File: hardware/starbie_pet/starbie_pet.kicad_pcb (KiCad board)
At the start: 2 copper layers, 11 parts, among them J1 Conn_01x04_Pin, J2 Conn_01x08_Pin, SW1 SW_Push, SW2 SW_Push, U1 XIAO-ESP32-C3-SMD, U2 DHT11

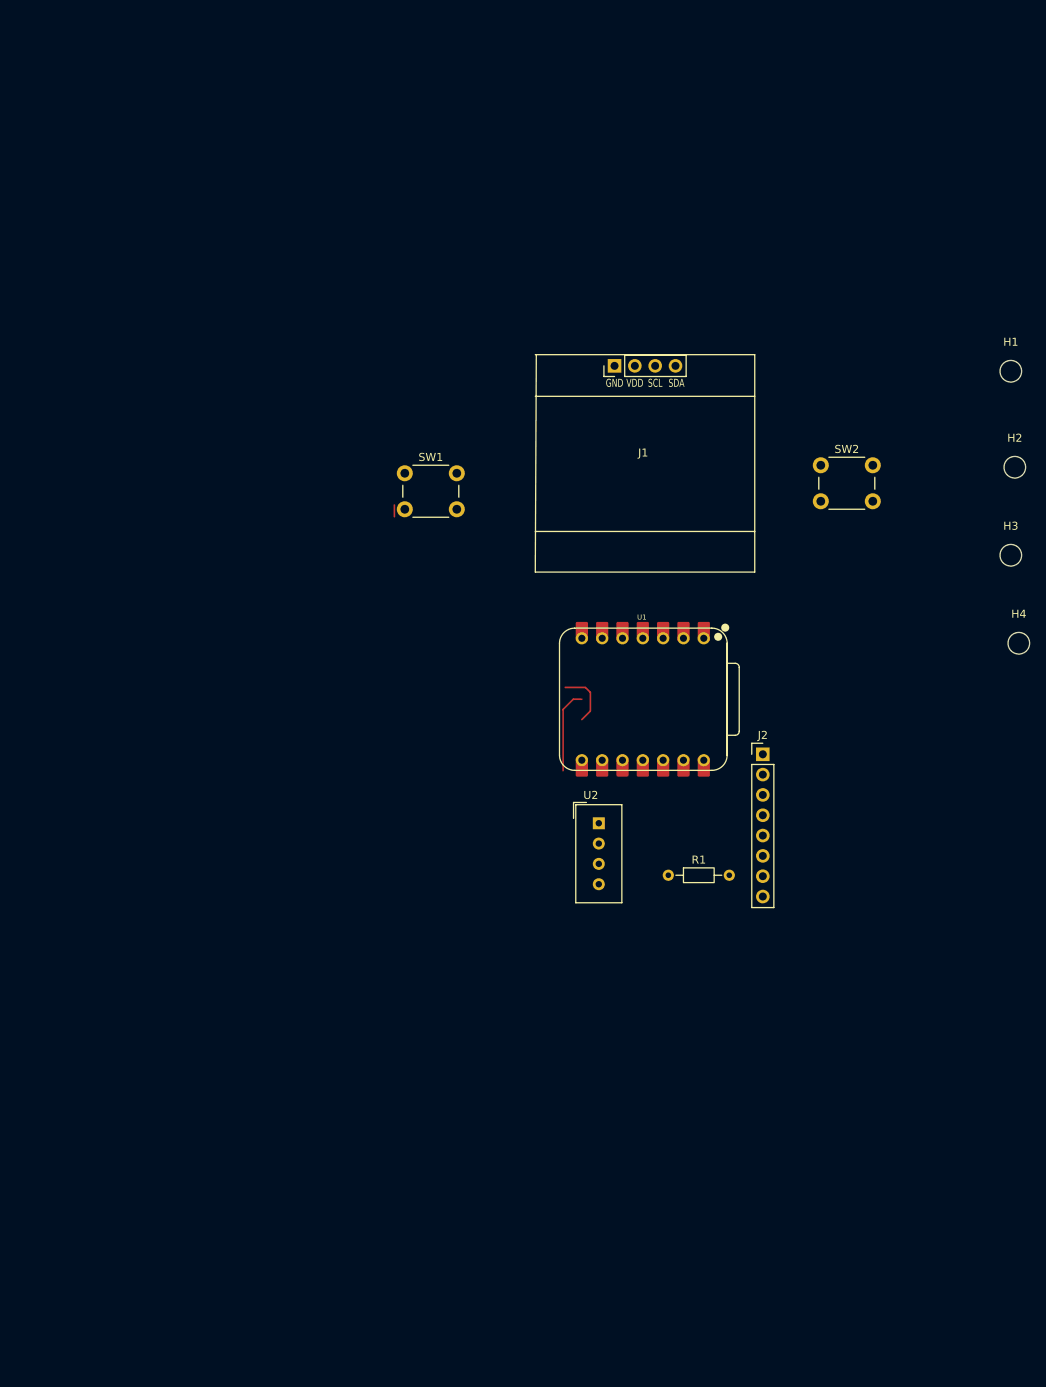
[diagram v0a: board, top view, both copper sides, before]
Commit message: before scaling
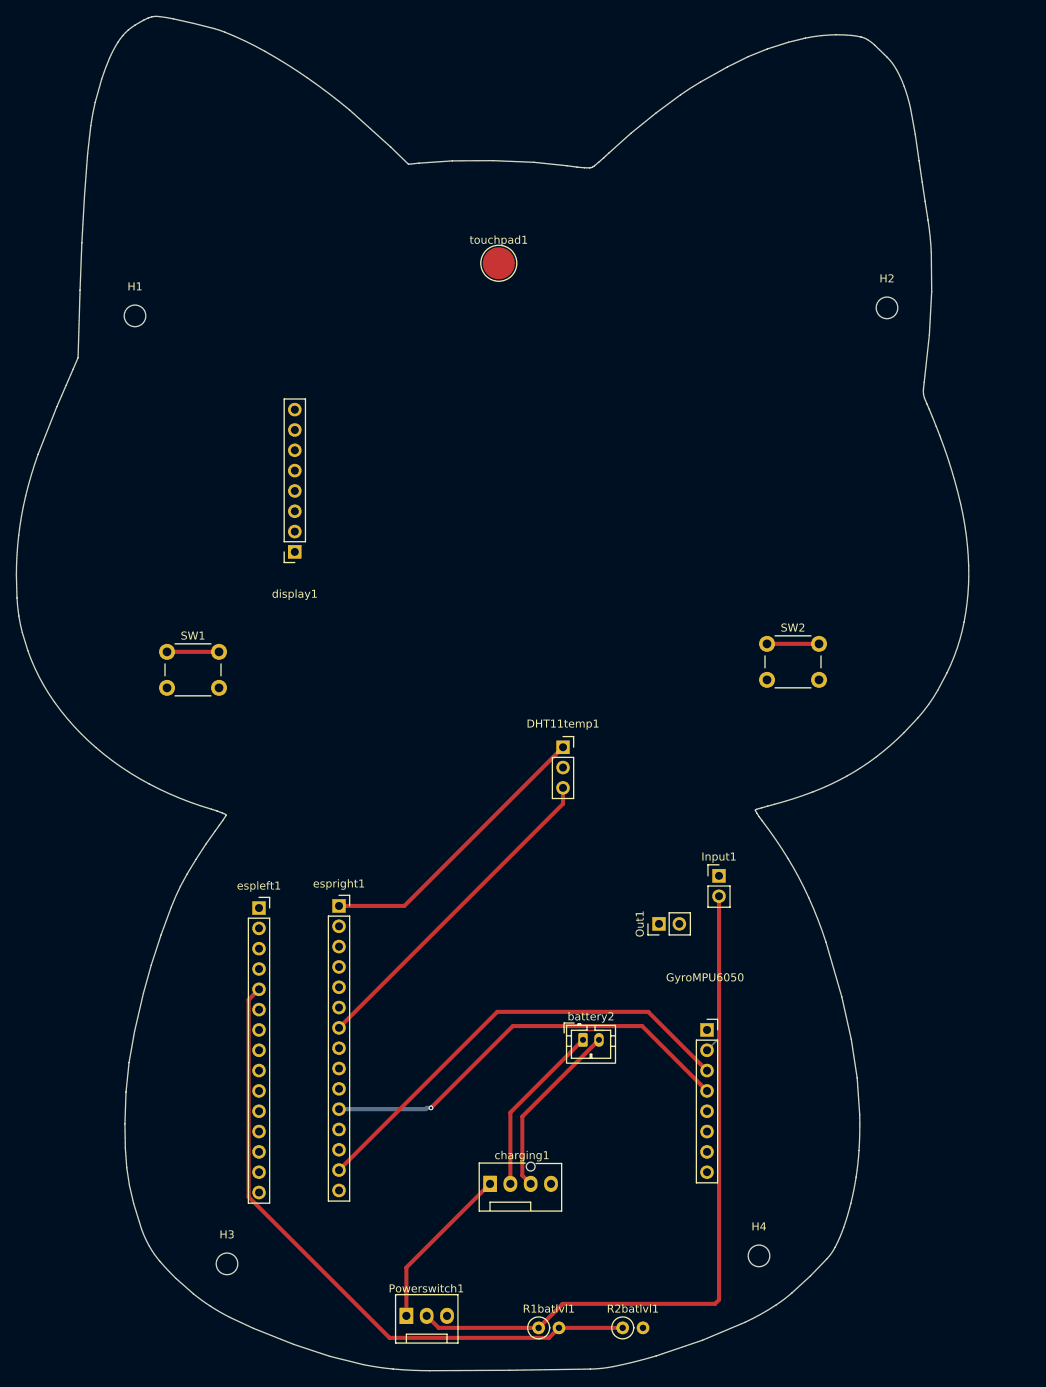
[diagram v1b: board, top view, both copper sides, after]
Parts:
- removed J1: Conn_01x04_Pin, Imported Parts:Display_128x64_096_I2C
- removed J2: Conn_01x08_Pin, Connector_PinHeader_2.54mm:PinHeader_1x08_P2.54mm_Vertical
- removed R1: 10k, Resistor_THT:R_Axial_DIN0204_L3.6mm_D1.6mm_P7.62mm_Horizontal
- removed U1: XIAO-ESP32-C3-SMD, Seeed_Studio_XIAO_Series:XIAO-ESP32-C6-DIP
- removed U2: DHT11, Sensor:Aosong_DHT11_5.5x12.0_P2.54mm
- added DHT11temp1: Conn_01x03_Socket, Connector_PinSocket_2.54mm:PinSocket_1x03_P2.54mm_Vertical, F.Cu at (134.0, 111.0)
- added GyroMPU6050: Conn_01x08_Socket, Connector_PinSocket_2.54mm:PinSocket_1x08_P2.54mm_Vertical, F.Cu at (152.0, 146.3)
- added Input1: Conn_01x02_Socket, Connector_PinHeader_2.54mm:PinHeader_1x02_P2.54mm_Vertical, F.Cu at (153.5, 127.1)
- added Out1: Conn_01x02_Socket, Connector_PinHeader_2.54mm:PinHeader_1x02_P2.54mm_Vertical, F.Cu at (146.0, 133.1)
- added Powerswitch1: SW_SPST, Connector:FanPinHeader_1x03_P2.54mm_Vertical, F.Cu at (114.4, 182.1)
- added R1batlvl1: R, Resistor_THT:R_Axial_DIN0207_L6.3mm_D2.5mm_P2.54mm_Vertical, F.Cu at (131.0, 183.6)
- added R2batlvl1: R, Resistor_THT:R_Axial_DIN0207_L6.3mm_D2.5mm_P2.54mm_Vertical, F.Cu at (141.5, 183.6)
- added battery2: Conn_01x02_Socket, Connector_JST:JST_PH_B2B-PH-K_1x02_P2.00mm_Vertical, F.Cu at (136.5, 147.6)
- added charging1: Conn_01x04_Socket, Connector:FanPinHeader_1x04_P2.54mm_Vertical, F.Cu at (124.9, 165.6)
- added display1: Conn_01x08_Socket, Connector_PinSocket_2.54mm:PinSocket_1x08_P2.54mm_Vertical, F.Cu at (100.5, 86.6)
- added espleft1: Conn_01x15_Socket, Connector_PinSocket_2.54mm:PinSocket_1x15_P2.54mm_Vertical, F.Cu at (96.0, 131.1)
- added espright1: Conn_01x15_Socket, Connector_PinSocket_2.54mm:PinSocket_1x15_P2.54mm_Vertical, F.Cu at (106.0, 130.8)
- added touchpad1: Conn_01x01, TestPoint:TestPoint_Pad_D4.0mm, F.Cu at (126.0, 50.5)
- SW1, SW2: footprint Button_Switch_THT:SW_PUSH_6mm_H5mm -> Button_Switch_THT:SW_PUSH_6mm
- moved H3 132.1 mm to (92.0, 175.6)
- moved H1 109.7 mm to (80.5, 57.1)
- moved H4 83.2 mm to (158.5, 174.6)
- moved SW1 37.2 mm to (84.5, 99.1)
- moved H2 25.5 mm to (174.5, 56.1)
- moved SW2 23.3 mm to (159.5, 98.1)
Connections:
- SW1 pad 1: GND -> /BUTTON
- SW1 pad 2: Net-(U1-D2) -> GND
- SW2 pad 1: GND -> /Button2
- SW2 pad 2: Net-(U1-D1) -> GND
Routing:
- net /Vbat: track 0.00 -> 89.1 mm
- net /Bat_sense: track 0.00 -> 81.1 mm
- net /I2C_SCL: track 0.00 -> 57.2 mm
- net /I2C_SDA: track 0.00 -> 53.7 mm, vias 0 -> 1
- net /DHT_DATA: track 0.00 -> 41.6 mm
- net +3V3: track 0.00 -> 36.2 mm
- net /Bat_neg: track 0.00 -> 22.4 mm
- net /Bat_pos: track 0.00 -> 21.8 mm
- net /CHG_OUT: track 0.00 -> 20.8 mm
- net /DHT11 DATA: track 10.5 -> 0.00 mm
- net +3.3V: track 7.25 -> 0.00 mm
- net /Button2: track 0.00 -> 6.50 mm
- net /BUTTON: track 0.00 -> 6.50 mm
- net +5V: track 0.00 -> 3.26 mm
- net GND: track 0.00 -> 1.63 mm
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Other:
- board outline added: 119.1 x 169.3 mm

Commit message: Add PCB files
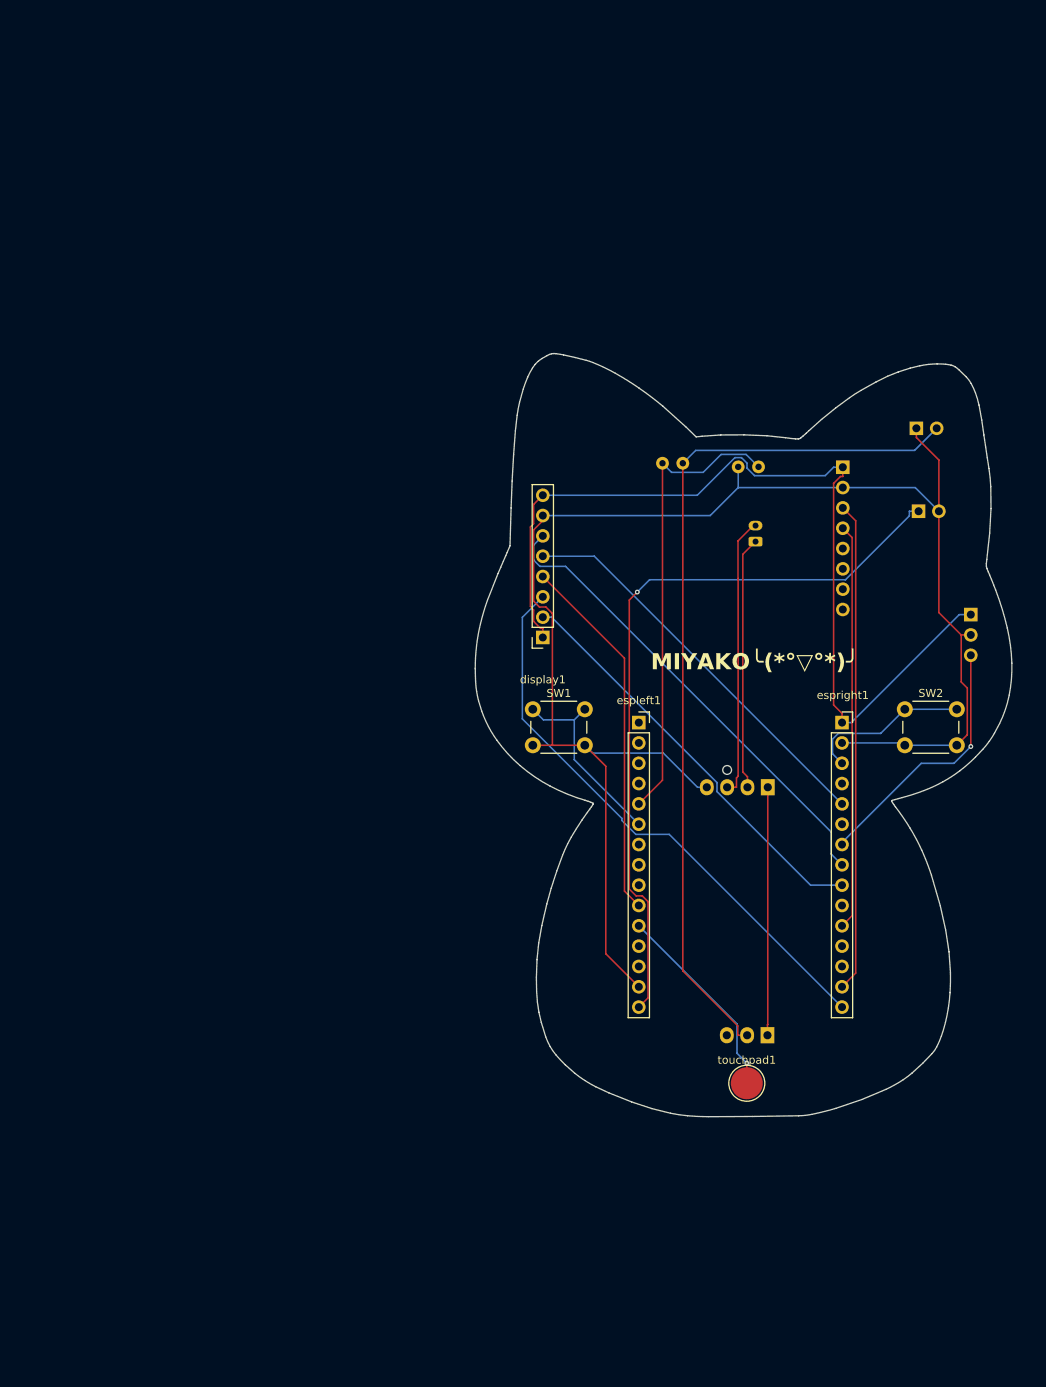
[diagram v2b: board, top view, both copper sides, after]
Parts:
- removed H1, H2, H3, H4: MountingHole, MountingHole:MountingHole_2.7mm_M2.5
- DHT11temp1, GyroMPU6050, Input1, Out1, Powerswitch1, R1batlvl1, R2batlvl1, battery2, charging1: moved to B.Cu
- moved R1batlvl1 109.6 mm to (149.0, 75.5), turned to 180 degrees
- moved R2batlvl1 109.0 mm to (158.5, 76.0), turned to 180 degrees
- moved touchpad1 107.1 mm to (157.0, 153.0)
- moved GyroMPU6050 72.4 mm to (169.0, 76.0), turned to 180 degrees
- moved espright1 66.9 mm to (168.9, 107.9)
- moved battery2 65.9 mm to (158.1, 85.3), turned to 90 degrees
- moved Input1 61.1 mm to (178.2, 71.1), turned to -90 degrees
- moved Out1 60.9 mm to (178.5, 81.5), turned to -90 degrees
- moved charging1 60.5 mm to (159.6, 116.0), turned to 180 degrees
- moved Powerswitch1 57.2 mm to (159.6, 147.0), turned to 180 degrees
- moved DHT11temp1 53.6 mm to (185.0, 94.4), turned to 180 degrees
- moved espleft1 52.8 mm to (143.5, 107.9)
- moved SW1 46.3 mm to (130.2, 106.2)
- moved display1 32.8 mm to (131.5, 97.3)
- moved SW2 19.1 mm to (176.8, 106.2)
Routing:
- net GND: track 1.63 -> 200.8 mm
- net +5V: track 3.26 -> 93.9 mm, vias 0 -> 1
- net +3V3: track 36.2 -> 115.1 mm
- net /SPI_MOSI: track 0.00 -> 71.3 mm
- net /TFT_CS: track 0.00 -> 59.5 mm
- net /SPI_CLK: track 0.00 -> 51.9 mm
- net /TFT_RST: track 0.00 -> 50.2 mm
- net /TFT_DC: track 0.00 -> 46.1 mm
- net /TOUCH: track 0.00 -> 25.3 mm, vias 0 -> 1
- net /Bat_sense: track 81.1 -> 57.9 mm
- net /Vbat: track 89.1 -> 109.1 mm
- net /BUTTON: track 6.50 -> 24.0 mm
- net /Button2: track 6.50 -> 20.6 mm
- net /Bat_neg: track 22.4 -> 35.0 mm
- net /CHG_OUT: track 20.8 -> 31.0 mm
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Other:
- board size 119.1 x 169.3 mm -> 67.1 x 95.4 mm
- board text added: "MIYAKO╰(*°▽°*)╯"

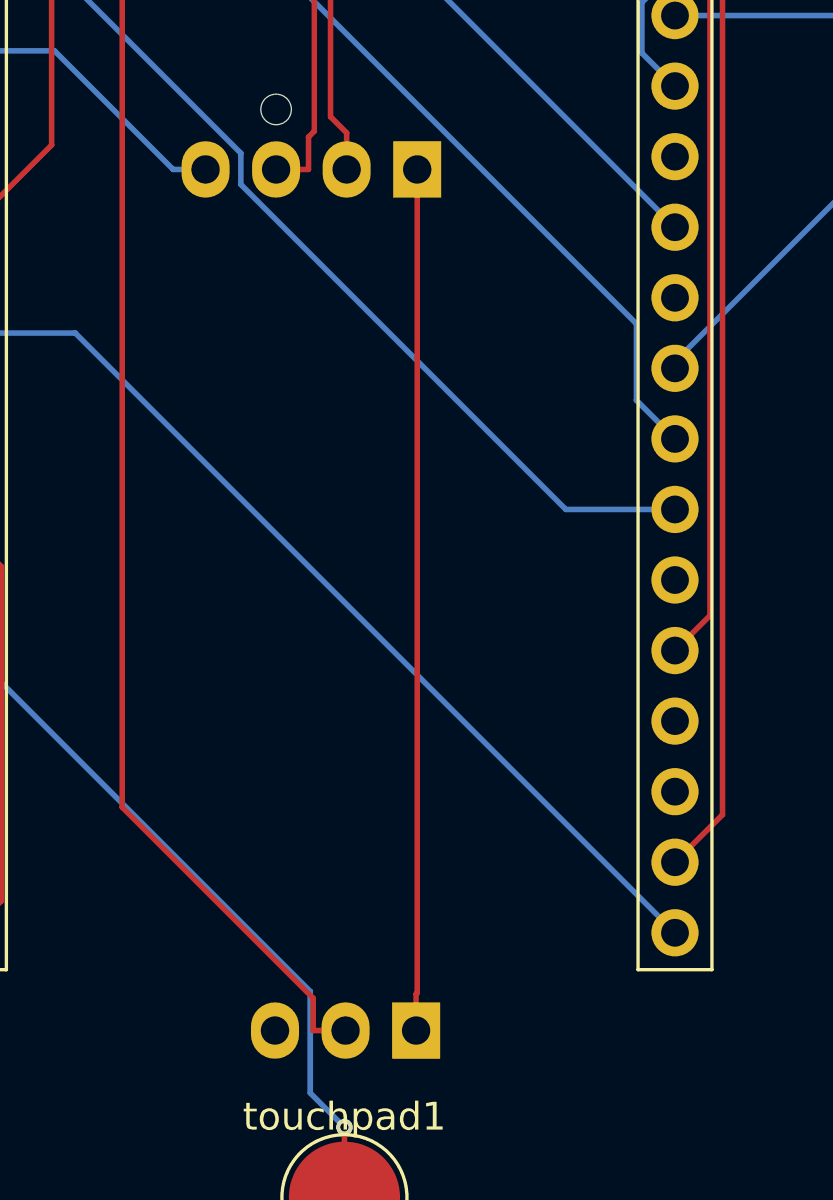
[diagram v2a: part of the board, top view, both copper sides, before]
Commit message: Update PCB traces and layout
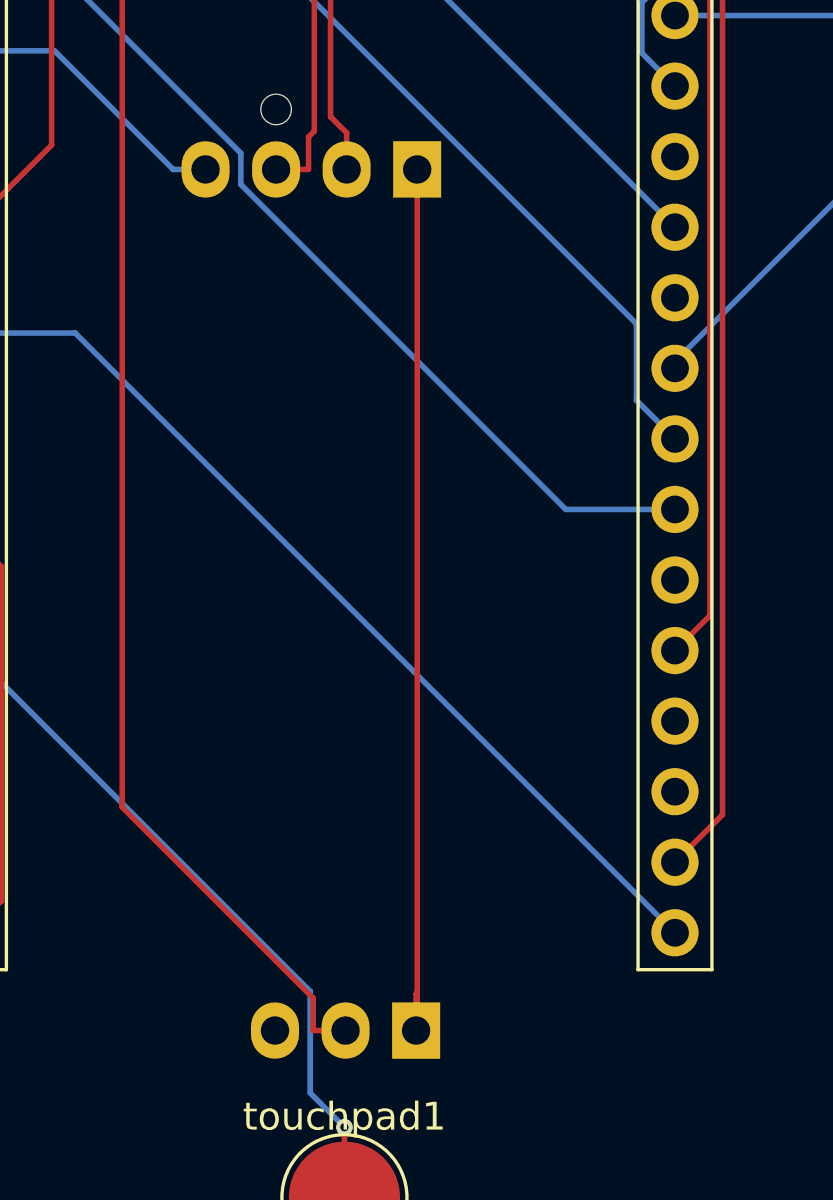
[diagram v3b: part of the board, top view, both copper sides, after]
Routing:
- net /CHG_OUT: track 31.0 -> 32.4 mm
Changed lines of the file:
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@@
 	)
 	(segment
-		(start 159.62 145.6433)
-		(end 159.62 116)
+		(start 159.62 116)
+		(end 159.62 146.96)
 		(width 0.2)
 		(layer "F.Cu")
+		(net "/CHG_OUT")
+	)
+	(segment
+		(start 159.62 146.96)
+		(end 159.58 147)
+		(width 0.2)
+		(layer "F.Cu")
